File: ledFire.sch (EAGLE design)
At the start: 29 parts, among them Q1 MUN5235DW1T1G, Q2 MUN5235DW1T1G, U1 MCP1640, U2 ATtiny84A-SSU

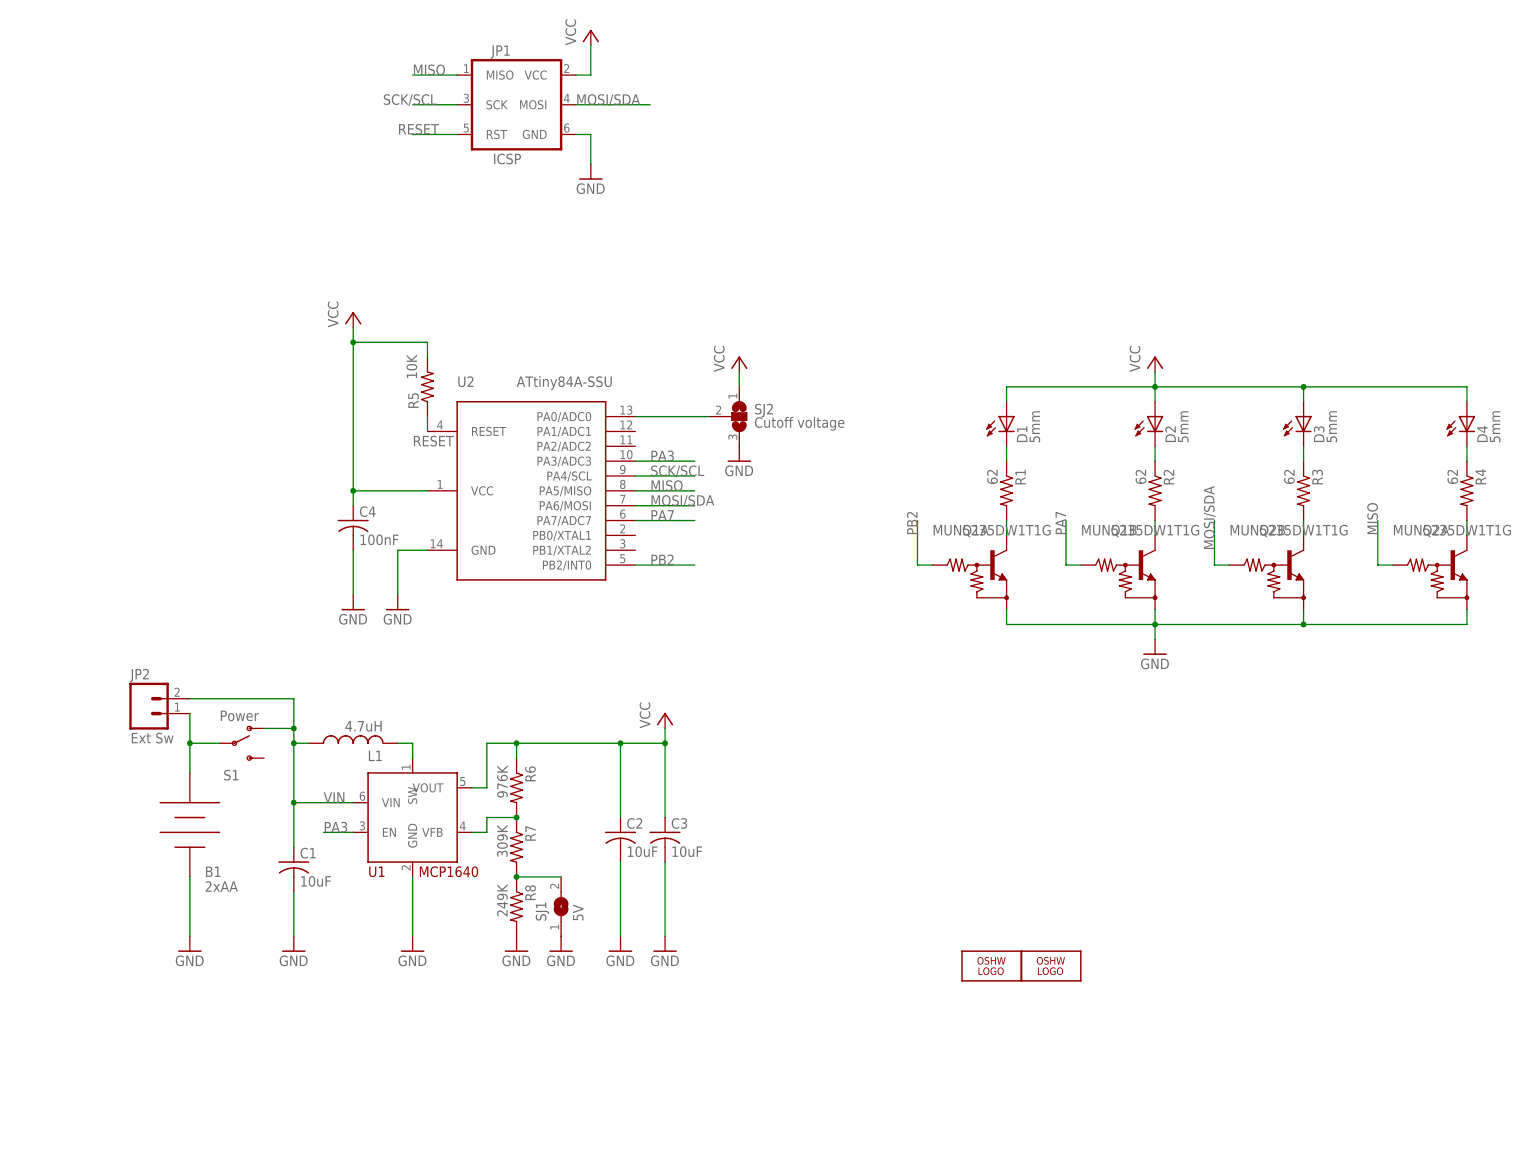
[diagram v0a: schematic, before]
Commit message: Update board and schematic images.
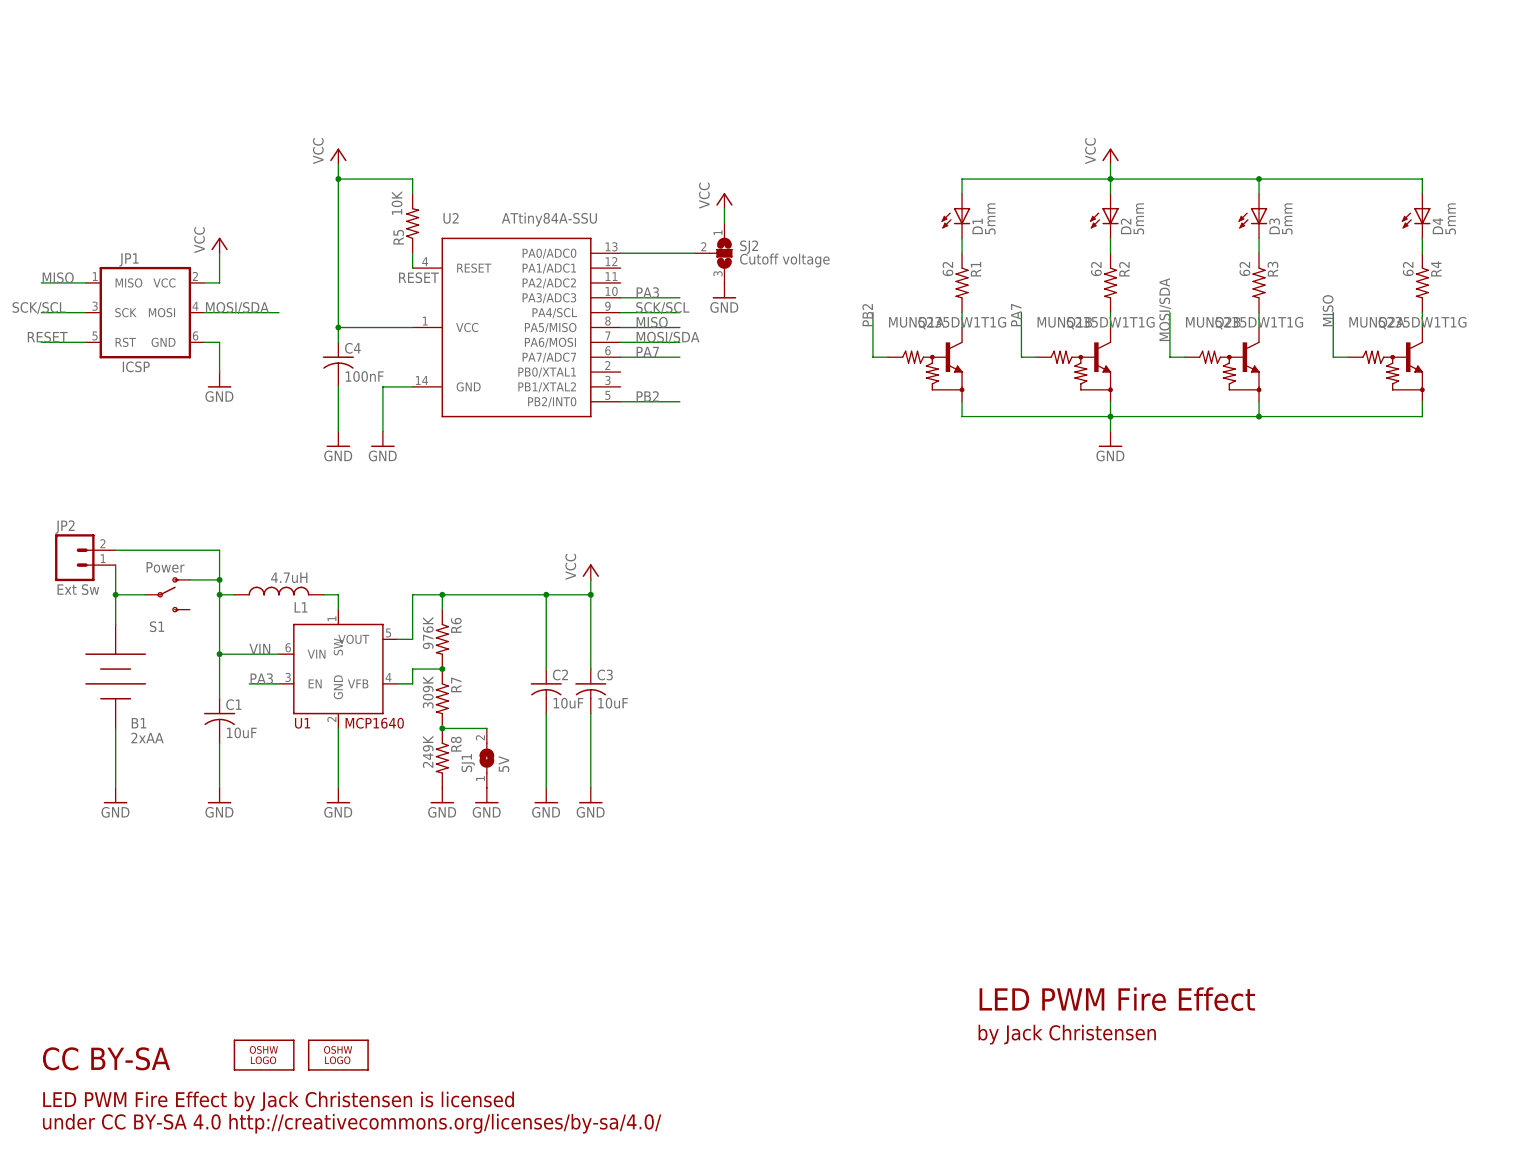
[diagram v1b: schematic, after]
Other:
- note added: "CC BY-SA"
- note added: "LED PWM Fire Effect"
- note added: "LED PWM Fire Effect by Jack Christensen is licensed under CC BY-SA 4.0 http://creativecommons.org/licenses/by-sa/4.0/"
- note added: "by Jack Christensen"
- moved on the sheet: B1, C1, C2, C3, C4, D1, D2, D3, D4, JP1, JP2, L1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
